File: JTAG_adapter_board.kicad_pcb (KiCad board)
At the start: 2 copper layers, 24.1 x 25.4 mm, 3 parts, among them J1 JTAG conn, J2 RJ11

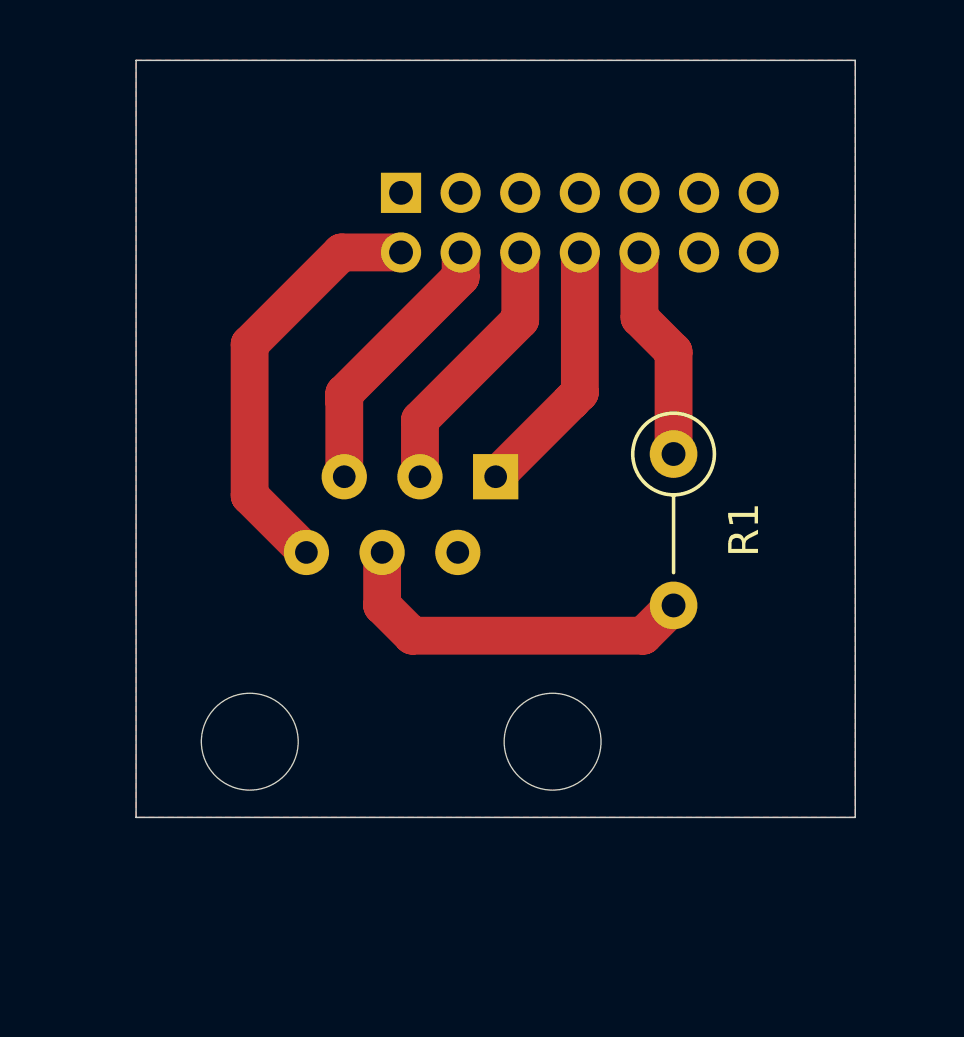
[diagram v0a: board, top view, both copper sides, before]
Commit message: Edits from keith, ready for fab
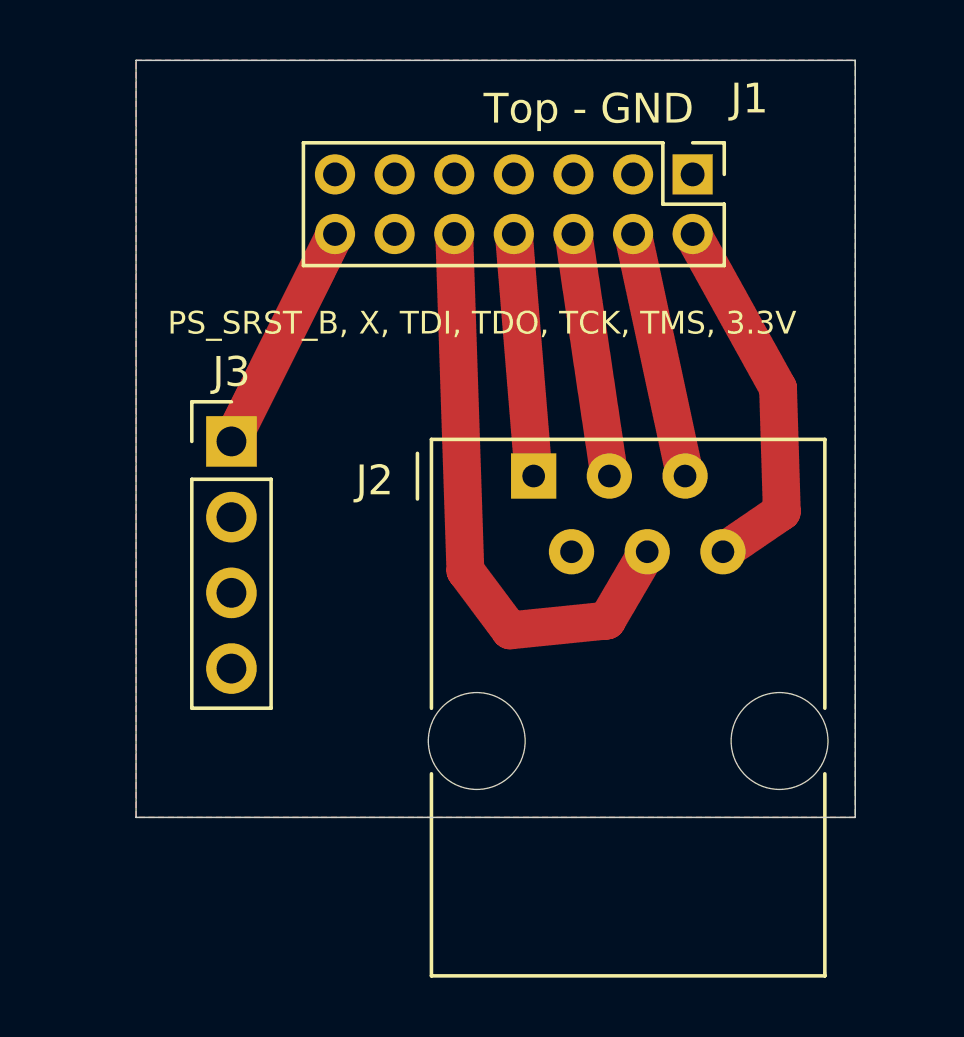
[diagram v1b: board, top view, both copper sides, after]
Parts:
- removed R1: 0hms, Resistor_THT:R_Axial_DIN0207_L6.3mm_D2.5mm_P5.08mm_Vertical
- added G***: LOGO, Coolsilks:jtag_bitmpa_rev1, B.Cu at (167.1, 88.2)
- added J3: P_SRST_breakout, Connector_PinHeader_2.54mm:PinHeader_1x04_P2.54mm_Vertical, F.Cu at (157.5, 87.1)
- J1, J2: moved to F.Cu
- moved J1 9.80 mm to (173.0, 78.1)
- moved J2 1.28 mm to (167.6, 88.2), turned to 0 degrees
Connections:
- J1 pad 6: (no net) -> GND
- J1 pad 7: (no net) -> GND
- J1 pad 8: (no net) -> /PS_SRST_B
- J1 pad 9: (no net) -> unconnected-(J1-Pad9)
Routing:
- net /PS_SRST_B: track 0.00 -> 7.78 mm
- net +3V3: track 14.1 -> 12.4 mm
- net /TMS: track 9.14 -> 8.31 mm
- net /TCK: track 8.92 -> 8.21 mm
- net /TD0: track 8.70 -> 8.15 mm
- added copper zone on B.Cu, net GND
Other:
- net class Default removed
- board text added: "PS_SRST_B, X, TDI, TDO, TCK, TMS, 3.3V"
- board text added: "Top - GND"
